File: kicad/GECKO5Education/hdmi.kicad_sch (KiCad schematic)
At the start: 24 parts, among them J2 HDMI_A, J6 Conn_01x06_Socket, J7 Conn_01x02_Pin, U16 LTC2632CTS8-LZ12TRMPBF, U17 MAX11666AUBV, U3 SII164CTG64, U6 LFE5U-85F-6BG381x

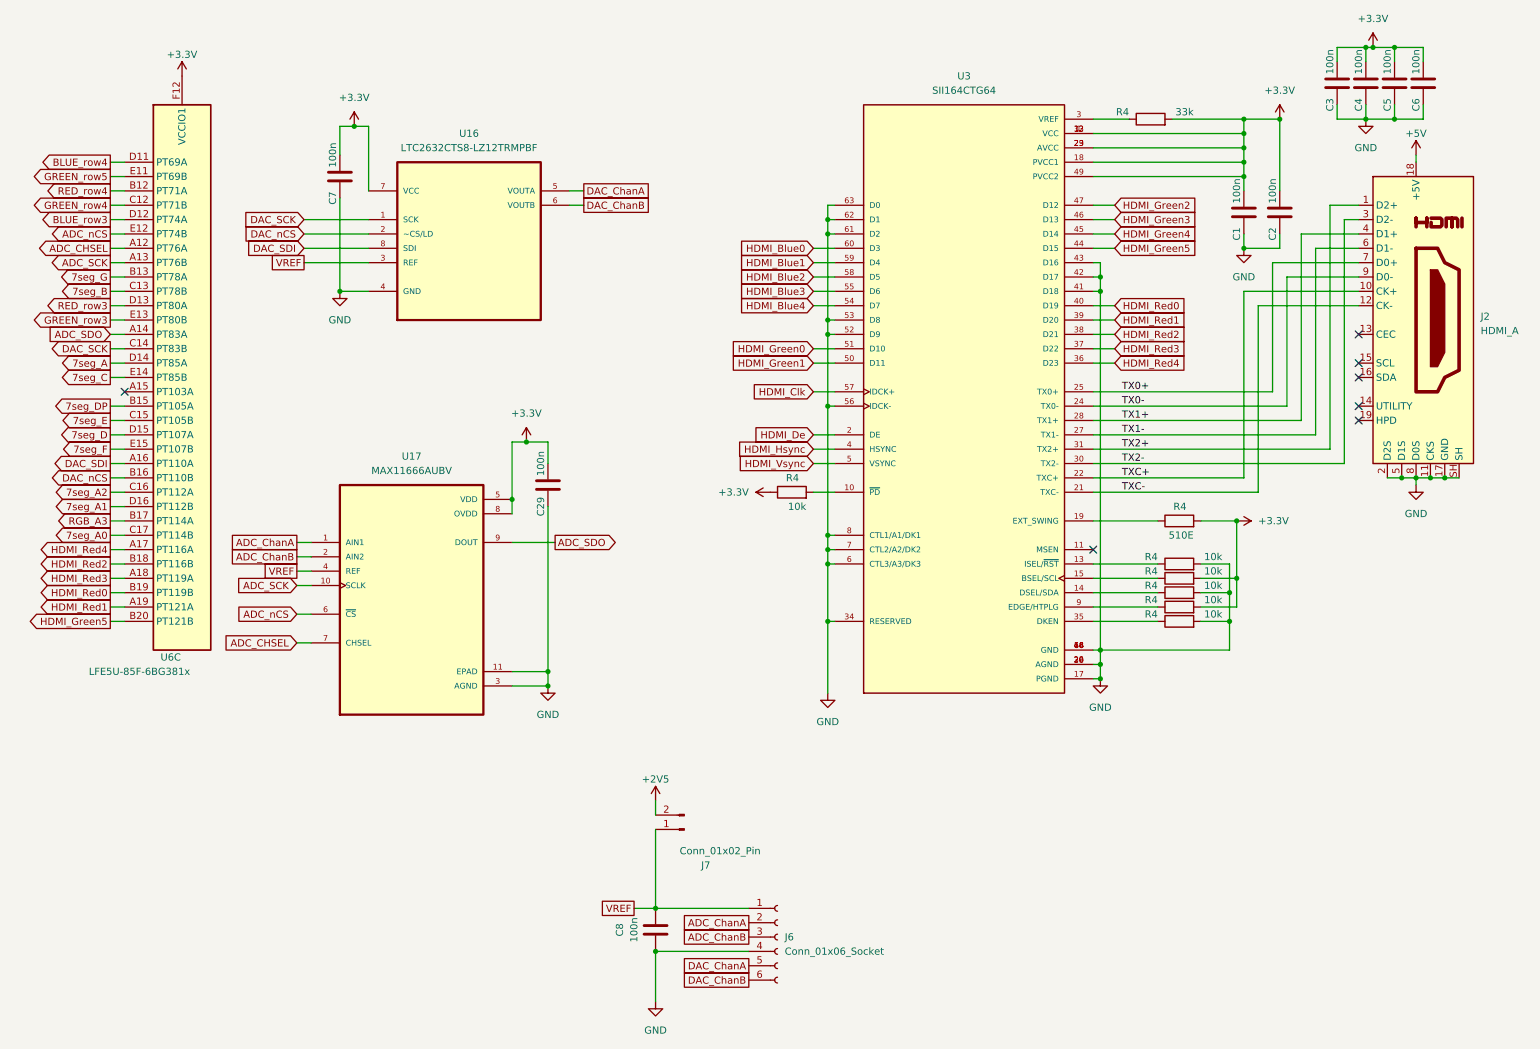
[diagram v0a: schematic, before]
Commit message: First version
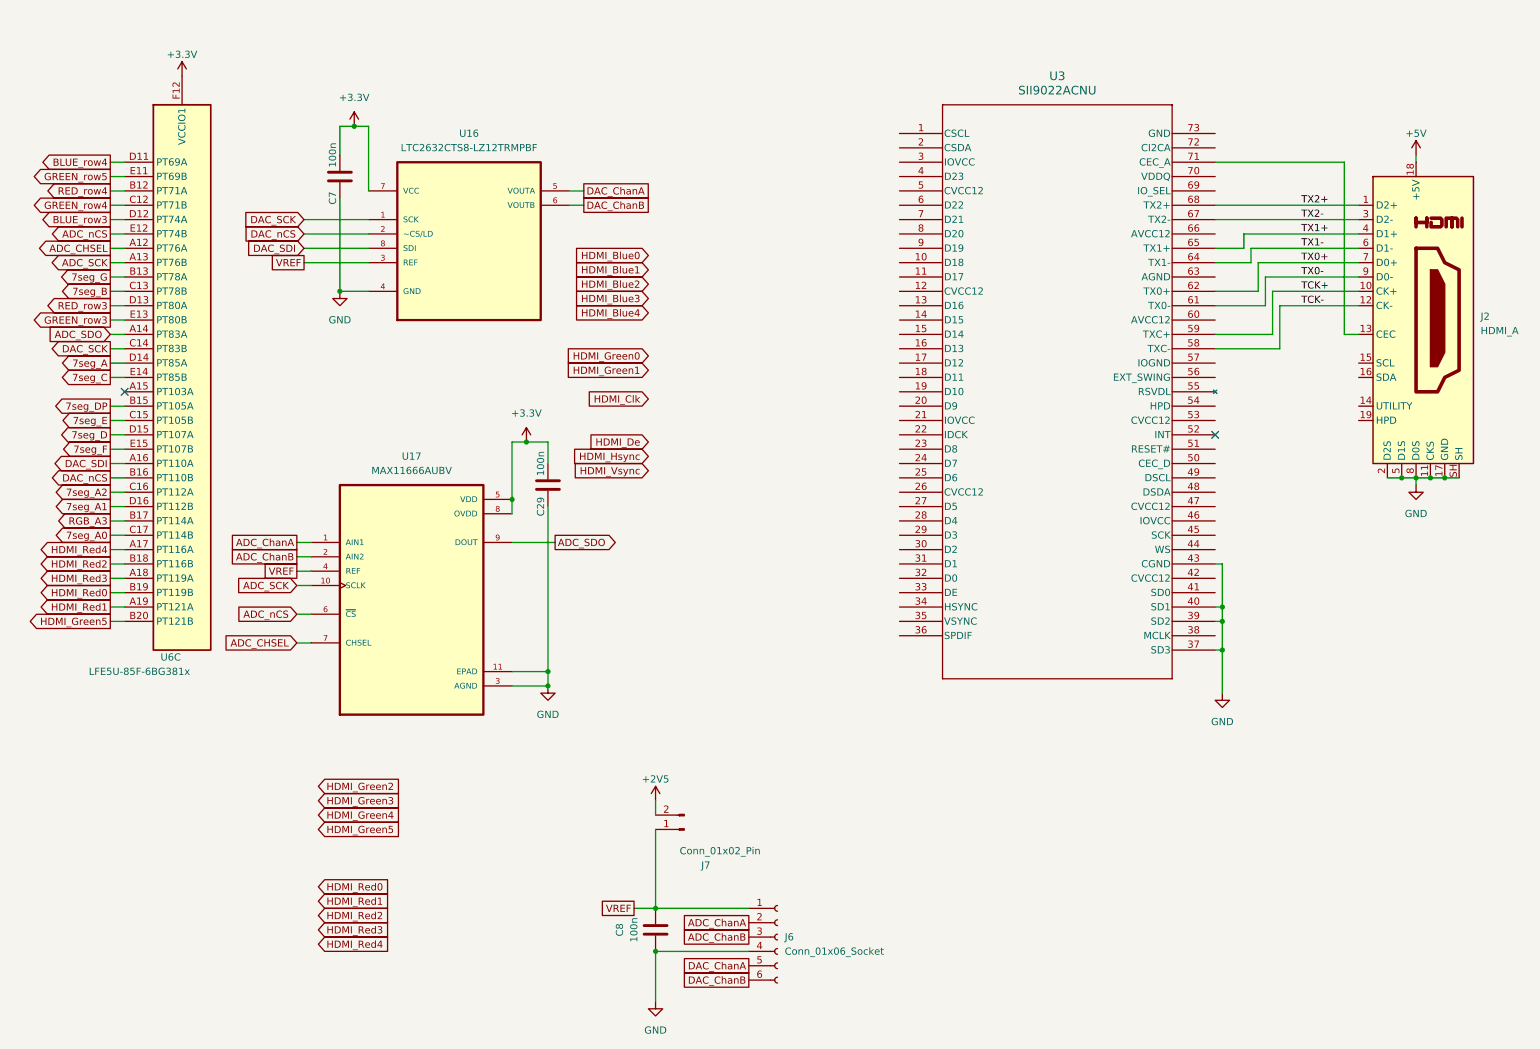
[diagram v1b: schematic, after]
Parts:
- removed C1, C2, C4, C5, C6: 100n, Capacitor_SMD:C_0402_1005Metric, symbol Device:C
- removed C3: 100n, Resistor_SMD:R_0402_1005Metric, symbol Device:C
- removed R4 (x6): 10k, Resistor_SMD:R_0402_1005Metric, symbol Device:R
- removed R4: 33k, Resistor_SMD:R_0402_1005Metric, symbol Device:R
- removed R4: 510E, Resistor_SMD:R_0402_1005Metric, symbol Device:R
- removed U3: SII164CTG64, gecko4education:QFP50P1200X1200X120-64N, symbol gecko5education:SII164CTG64
- added U3: SII9022ACNU, gecko4education:QFN72_10X10_LAT-M, symbol gecko5education:SII9022ACNU
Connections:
- net GND: now also U3.37 (SD3), U3.39 (SD2), U3.40 (SD1), U3.43 (CGND)
- net TX0+: now also U3.62 (TX0+)
- net TX0-: now also U3.61 (TX0-)
- net TX1+: now also U3.65 (TX1+)
- net TX1-: now also U3.64 (TX1-)
- net TX2+: now also U3.68 (TX2+)
- net TX2-: now also U3.67 (TX2-)
- net at J2.13 (CEC): now also U3.71 (CEC_A)
- net TXC+ renamed TCK+
- net TCK+: now also U3.59 (TXC+)
- net TXC- renamed TCK-
- net TCK-: now also U3.58 (TXC-)
- no-connect marks 7 -> 2
